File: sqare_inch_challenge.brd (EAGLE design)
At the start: 25.4 x 25.4 mm, 23 parts

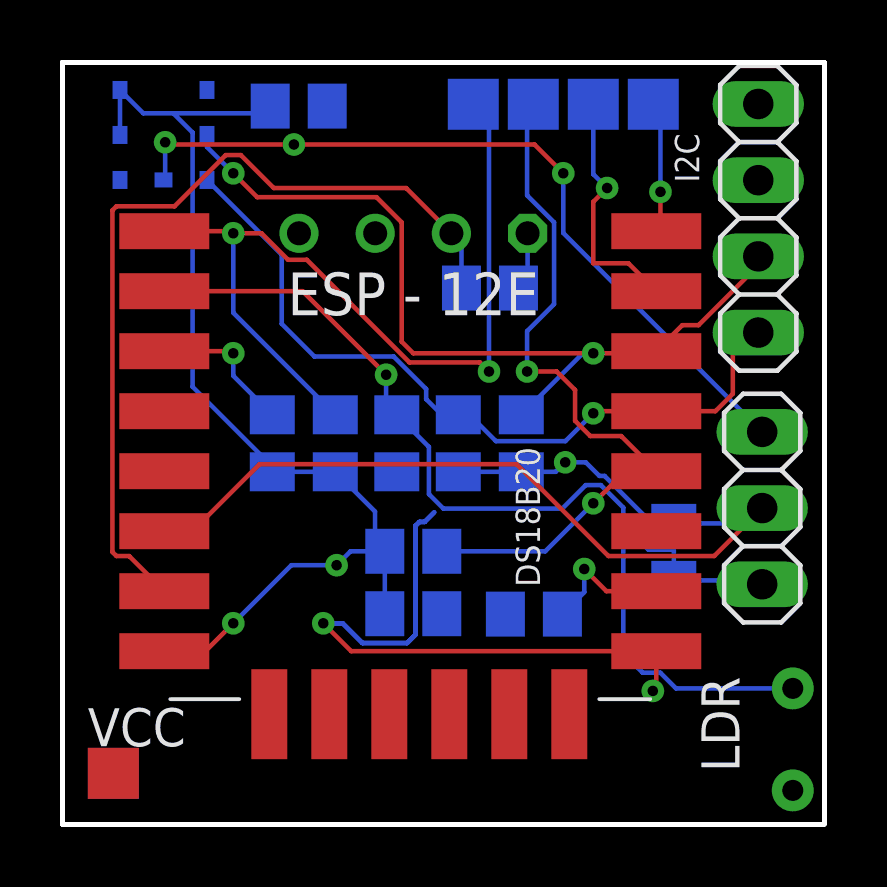
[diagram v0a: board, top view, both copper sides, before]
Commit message: Final Board Files
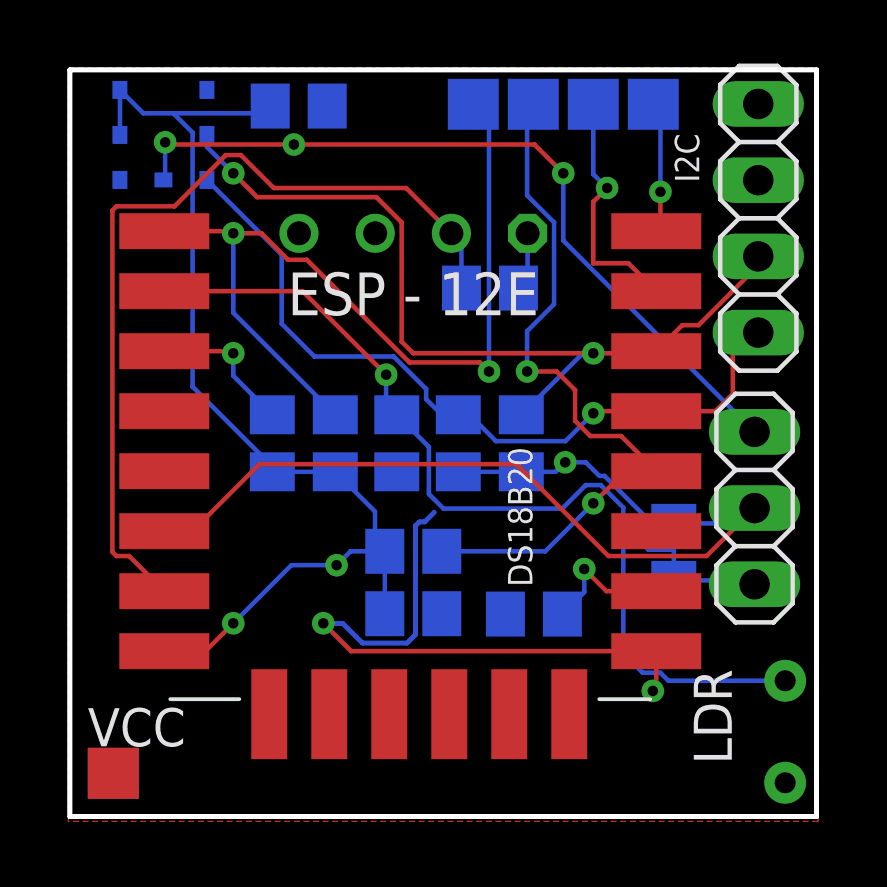
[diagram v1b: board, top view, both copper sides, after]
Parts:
- R7: value 10k -> 1k
- moved LDR 0.36 mm to (11.4, -9.62)
- moved DS18B20 0.25 mm to (10.4, -2.16)
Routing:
- net 1W: track 25.9 -> 25.4 mm
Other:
- board size 25.4 x 25.4 mm -> 24.9 x 24.9 mm
- board text added: "StanislavJochman"
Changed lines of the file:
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@@
 <setting verticaltext="up"/>
 </settings>
-<grid distance="1" unitdist="mm" unit="mm" style="lines" multiple="1" display="no" altdistance="5" altunitdist="mil" altunit="mm"/>
+<grid distance="0.01" unitdist="inch" unit="inch" style="lines" multiple="1" display="no" altdistance="5" altunitdist="mil" altunit="inch"/>
 <layers>
 <layer number="1" name="Top" color="4" fill="1" visible="yes" active="yes"/>
@@
 <board>
 <plain>
-<wire x1="-12.7" y1="-12.7" x2="-12.7" y2="12.7" width="0.1524" layer="46"/>
-<wire x1="-12.7" y1="12.7" x2="12.7" y2="12.7" width="0.1524" layer="46"/>
-<wire x1="12.7" y1="12.7" x2="12.7" y2="-12.7" width="0.1524" layer="46"/>
-<wire x1="12.7" y1="-12.7" x2="-12.7" y2="-12.7" width="0.1524" layer="46"/>
-<wire x1="-12.7" y1="-12.7" x2="12.7" y2="-12.7" width="0.1524" layer="20"/>
-<wire x1="12.7" y1="-12.7" x2="12.7" y2="12.7" width="0.1524" layer="20"/>
-<wire x1="12.7" y1="12.7" x2="-12.7" y2="12.7" width="0.1524" layer="20"/>
-<wire x1="-12.7" y1="12.7" x2="-12.7" y2="-12.7" width="0.1524" layer="20"/>
+<wire x1="-12.446" y1="-12.446" x2="-12.446" y2="12.446" width="0.1524" layer="46"/>
+<wire x1="-12.446" y1="12.446" x2="12.446" y2="12.446" width="0.1524" layer="46"/>
+<wire x1="12.446" y1="12.446" x2="12.446" y2="-12.446" width="0.1524" layer="46"/>
+<wire x1="12.446" y1="-12.446" x2="-12.446" y2="-12.446" width="0.1524" layer="46"/>
+<wire x1="-12.446" y1="-12.446" x2="12.446" y2="-12.446" width="0.1524" layer="20"/>
+<wire x1="12.446" y1="-12.446" x2="12.446" y2="12.446" width="0.1524" layer="20"/>
+<wire x1="12.446" y1="12.446" x2="-12.446" y2="12.446" width="0.1524" layer="20"/>
+<wire x1="-12.446" y1="12.446" x2="-12.446" y2="-12.446" width="0.1524" layer="20"/>
+<text x="0" y="-9" size="1.6" layer="28" rot="MR0" align="center">StanislavJochman</text>
 </plain>
 <attributes>
@@
 <attribute name="VALUE" x="2.553" y="4.588" size="0.8128" layer="28" rot="MR270"/>
 </element>
-<element name="LDR" library="Square_inch_Challange" package="T0-46-A10XX" package3d_urn="urn:adsk.eagle:package:22201/1" value="LDR" x="11.65" y="-9.87" smashed="yes" rot="R90">
-<attribute name="VALUE" x="9.873" y="-10.951" size="1.27" layer="25" rot="R90"/>
-</element>
-<element name="R7" library="rcl" library_urn="urn:adsk.eagle:library:334" package="R0805" package3d_urn="urn:adsk.eagle:package:23553/2" value="10k" x="-1.55" y="0" smashed="yes" rot="MR90">
+<element name="LDR" library="Square_inch_Challange" package="T0-46-A10XX" package3d_urn="urn:adsk.eagle:package:22201/1" value="LDR" x="11.396" y="-9.616" smashed="yes" rot="R90">
+<attribute name="VALUE" x="9.619" y="-10.697" size="1.27" layer="25" rot="R90"/>
+</element>
+<element name="R7" library="rcl" library_urn="urn:adsk.eagle:library:334" package="R0805" package3d_urn="urn:adsk.eagle:package:23553/2" value="1k" x="-1.55" y="0" smashed="yes" rot="MR90">
 <attribute name="SPICEPREFIX" value="R" x="-1.55" y="0" size="1.778" layer="28" rot="MR90" display="off"/>
 <attribute name="VALUE" x="-0.625" y="3.937" size="0.8128" layer="28" rot="MR270"/>
@@
 </element>
 <element name="GND" library="testpad" library_urn="urn:adsk.eagle:library:385" package="TP17SQ" package3d_urn="urn:adsk.eagle:package:27977/1" value="GND" x="-11" y="-11" smashed="yes" rot="MR0">
-<attribute name="NAME" x="-6.2461" y="-11.5301" size="1.27" layer="26" rot="MR0"/>
+<attribute name="NAME" x="-6.5001" y="-11.6571" size="1.27" layer="26" rot="MR0"/>
 <attribute name="TP_SIGNAL_NAME" value="" x="-11" y="-13.54" size="1" layer="38" rot="MR0"/>
 <attribute name="VALUE" x="-10.238" y="-11.889" size="0.0254" layer="28" rot="MR0"/>
@@
 <attribute name="VALUE" x="-0.778" y="4.698" size="0.8128" layer="28" rot="MR0"/>
 </element>
-<element name="DS18B20" library="pinhead" library_urn="urn:adsk.eagle:library:325" package="1X03" package3d_urn="urn:adsk.eagle:package:22458/2" value="" x="10.63" y="-2.16" smashed="yes" rot="R270">
-<attribute name="NAME" x="2.4118" y="-0.1308" size="0.8128" layer="25" ratio="10" rot="R270"/>
-<attribute name="VALUE" x="7.455" y="1.65" size="1.27" layer="27" rot="R270"/>
+<element name="DS18B20" library="pinhead" library_urn="urn:adsk.eagle:library:325" package="1X03" package3d_urn="urn:adsk.eagle:package:22458/2" value="" x="10.376" y="-2.16" smashed="yes" rot="R270">
+<attribute name="NAME" x="2.1578" y="-0.1308" size="0.8128" layer="25" ratio="10" rot="R270"/>
+<attribute name="VALUE" x="7.201" y="1.65" size="1.27" layer="27" rot="R270"/>
 </element>
 </elements>
@@
 <contactref element="I2C" pad="2"/>
 <polygon width="0.1524" layer="16">
-<vertex x="-12.7" y="12.7"/>
-<vertex x="12.7" y="12.7"/>
-<vertex x="12.7" y="-12.7"/>
-<vertex x="-12.7" y="-12.7"/>
+<vertex x="-12.5" y="12.5"/>
+<vertex x="12.5" y="12.5"/>
+<vertex x="12.5" y="-12.5"/>
+<vertex x="-12.5" y="-12.5"/>
 </polygon>
 <contactref element="GND" pad="TP"/>
@@
 <wire x1="-0.9286" y1="-2.7553125" x2="-0.9286" y2="-6.3818875" width="0.1524" layer="16"/>
 <wire x1="-0.9286" y1="-6.3818875" x2="-1.2053125" y2="-6.6586" width="0.1524" layer="16"/>
-<wire x1="10.63" y1="0.38" x2="4" y2="7.01" width="0.1524" layer="16"/>
-<wire x1="4" y1="7.01" x2="4" y2="9" width="0.1524" layer="16"/>
+<wire x1="10.376" y1="0.38" x2="4" y2="6.756" width="0.1524" layer="16"/>
+<wire x1="4" y1="6.756" x2="4" y2="9" width="0.1524" layer="16"/>
 <via x="4" y="9" extent="1-16" drill="0.35"/>
 <wire x1="4" y1="9" x2="3.0406" y2="9.9594" width="0.1524" layer="1"/>
@@
 <wire x1="4.064" y1="-0.635" x2="4.75" y2="-0.635" width="0.1524" layer="16"/>
 <contactref element="DS18B20" pad="3"/>
-<wire x1="7.685" y1="-4.57" x2="10.5" y2="-4.57" width="0.1524" layer="16"/>
-<wire x1="10.5" y1="-4.57" x2="10.63" y2="-4.7" width="0.1524" layer="16"/>
+<wire x1="7.685" y1="-4.57" x2="10.246" y2="-4.57" width="0.1524" layer="16"/>
+<wire x1="10.246" y1="-4.57" x2="10.376" y2="-4.7" width="0.1524" layer="16"/>
 <wire x1="7.685" y1="-3.57" x2="7.685" y2="-4.57" width="0.1524" layer="16"/>
 <wire x1="4.75" y1="-0.635" x2="5.2034" y2="-1.0884" width="0.1524" layer="16"/>
@@
 <wire x1="6.7064" y1="-2.41719375" x2="6.7064" y2="-3.4146875" width="0.1524" layer="16"/>
 <polygon width="0.1524" layer="1">
-<vertex x="-12.7" y="12.7"/>
-<vertex x="12.7" y="12.7"/>
-<vertex x="12.7" y="-12.7"/>
-<vertex x="-12.7" y="-12.7"/>
+<vertex x="-12.5" y="12.5"/>
+<vertex x="12.5" y="12.5"/>
+<vertex x="12.5" y="-12.6"/>
+<vertex x="-12.5" y="-12.6"/>
 </polygon>
 <wire x1="-7" y1="-6" x2="-5.064" y2="-4.064" width="0.1524" layer="16"/>
@@
 <contactref element="U1" pad="GPIO12"/>
 <contactref element="R8" pad="1"/>
-<wire x1="7.685" y1="-2.67" x2="10.12" y2="-2.67" width="0.1524" layer="16"/>
-<wire x1="10.12" y1="-2.67" x2="10.63" y2="-2.16" width="0.1524" layer="16"/>
+<wire x1="7.685" y1="-2.67" x2="9.866" y2="-2.67" width="0.1524" layer="16"/>
+<wire x1="9.866" y1="-2.67" x2="10.376" y2="-2.16" width="0.1524" layer="16"/>
 <wire x1="-8.36105625" y1="-2.93" x2="-9.3" y2="-2.93" width="0.1524" layer="1"/>
 <wire x1="-6.12625625" y1="-0.6952" x2="-8.36105625" y2="-2.93" width="0.1524" layer="1"/>
-<wire x1="9.0314" y1="-3.7586" x2="5.5053125" y2="-3.7586" width="0.1524" layer="1"/>
+<wire x1="8.7774" y1="-3.7586" x2="5.5053125" y2="-3.7586" width="0.1524" layer="1"/>
 <wire x1="5.5053125" y1="-3.7586" x2="2.4419125" y2="-0.6952" width="0.1524" layer="1"/>
 <wire x1="2.4419125" y1="-0.6952" x2="-6.12625625" y2="-0.6952" width="0.1524" layer="1"/>
-<wire x1="10.63" y1="-2.16" x2="9.0314" y2="-3.7586" width="0.1524" layer="1"/>
+<wire x1="10.376" y1="-2.16" x2="8.7774" y2="-3.7586" width="0.1524" layer="1"/>
 <contactref element="DS18B20" pad="2"/>
 </signal>
@@
 <wire x1="6" y1="-7" x2="6.6482" y2="-7.6482" width="0.1524" layer="16"/>
 <wire x1="6.6482" y1="-7.6482" x2="7.23635" y2="-7.6482" width="0.1524" layer="16"/>
-<wire x1="7.23635" y1="-7.6482" x2="7.75815" y2="-8.17" width="0.1524" layer="16"/>
-<wire x1="7.75815" y1="-8.17" x2="11.65" y2="-8.17" width="0.1524" layer="16"/>
+<wire x1="7.23635" y1="-7.6482" x2="7.50415" y2="-7.916" width="0.1524" layer="16"/>
+<wire x1="7.50415" y1="-7.916" x2="11.396" y2="-7.916" width="0.1524" layer="16"/>
 </signal>
 </signals>
